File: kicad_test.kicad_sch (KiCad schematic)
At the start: 7 parts, among them U1 ICM7555xP, U2 ICM7555xP

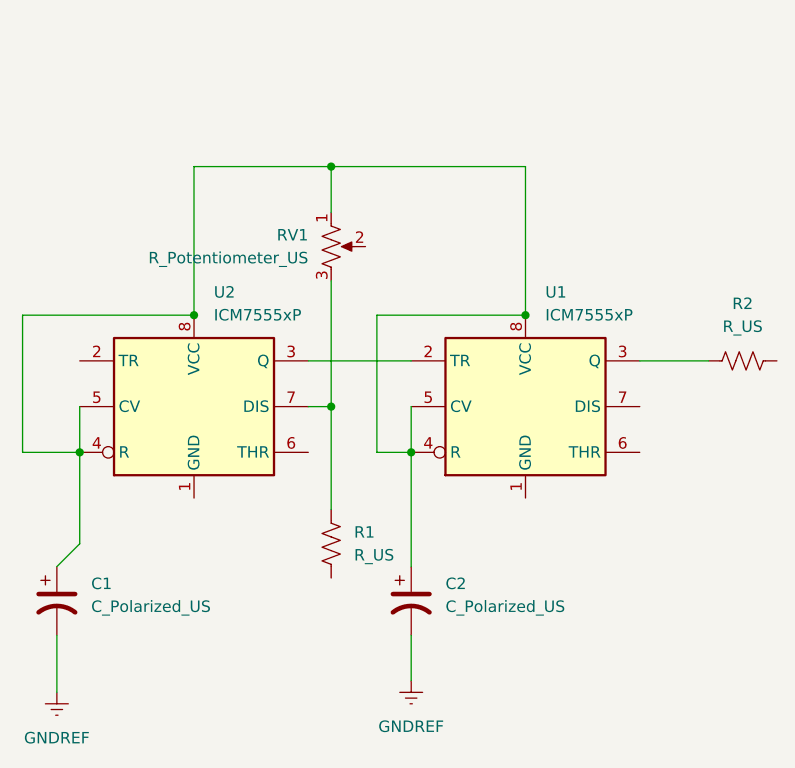
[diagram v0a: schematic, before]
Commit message: couple changes
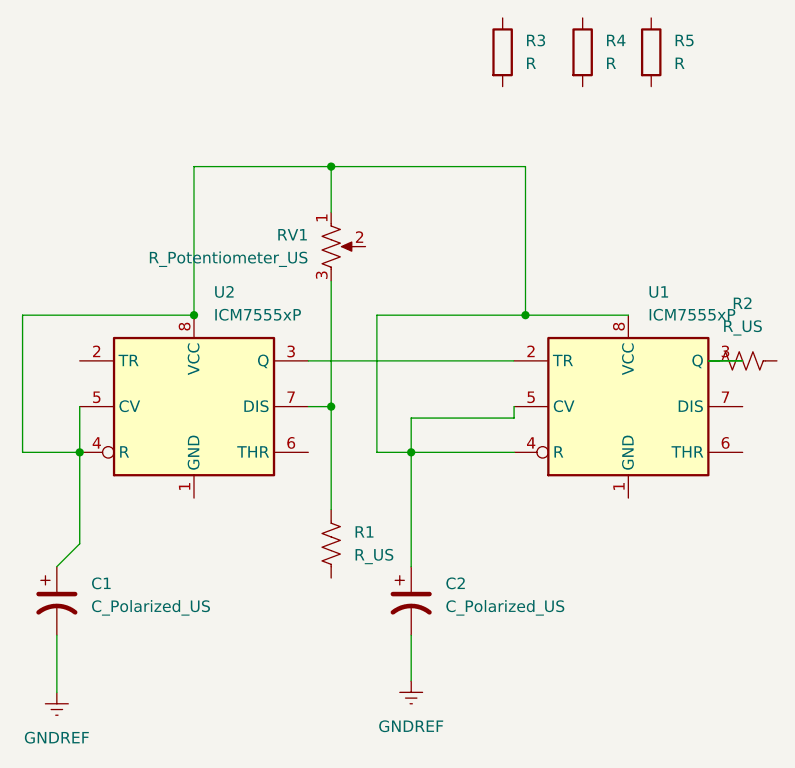
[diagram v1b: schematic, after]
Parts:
- added R3, R4, R5: R, symbol Device:R
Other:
- moved on the sheet: U1
